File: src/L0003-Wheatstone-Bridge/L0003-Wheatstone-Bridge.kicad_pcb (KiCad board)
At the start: 2 copper layers, 64.3 x 19.3 mm, 21 parts, among them P1 12V, P2 SULLINS_PPTC041LFBN-RC, P3 CON_39299043, P4 CON_39299043, U1 MCP1703T-4002E_DB

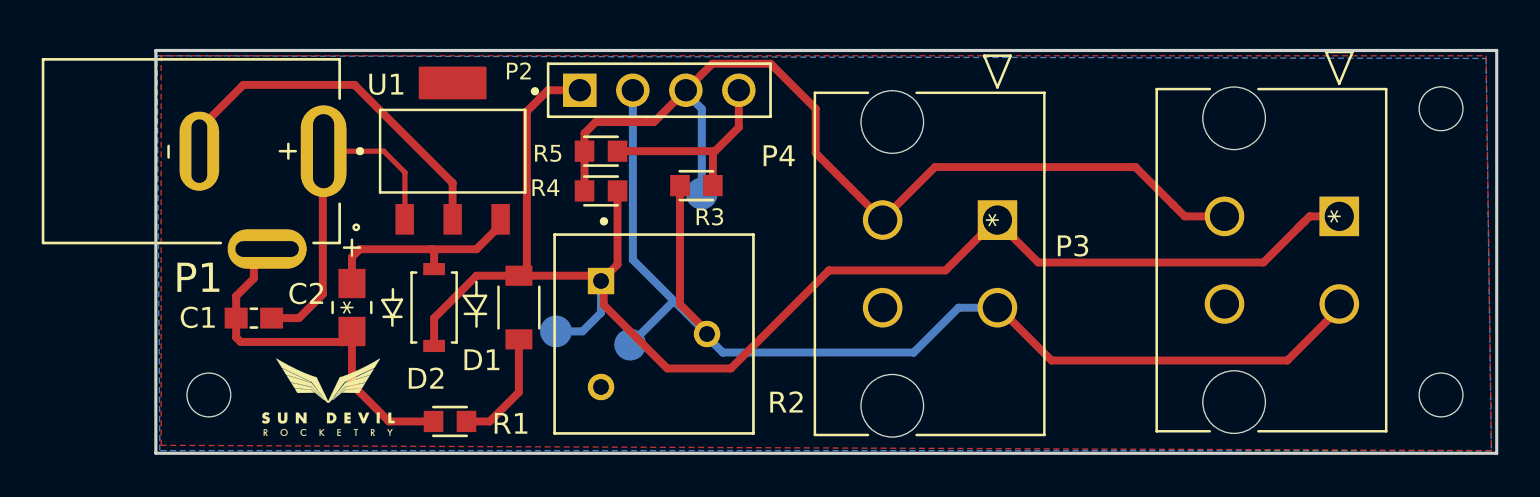
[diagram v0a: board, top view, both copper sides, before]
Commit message: routed rev 3
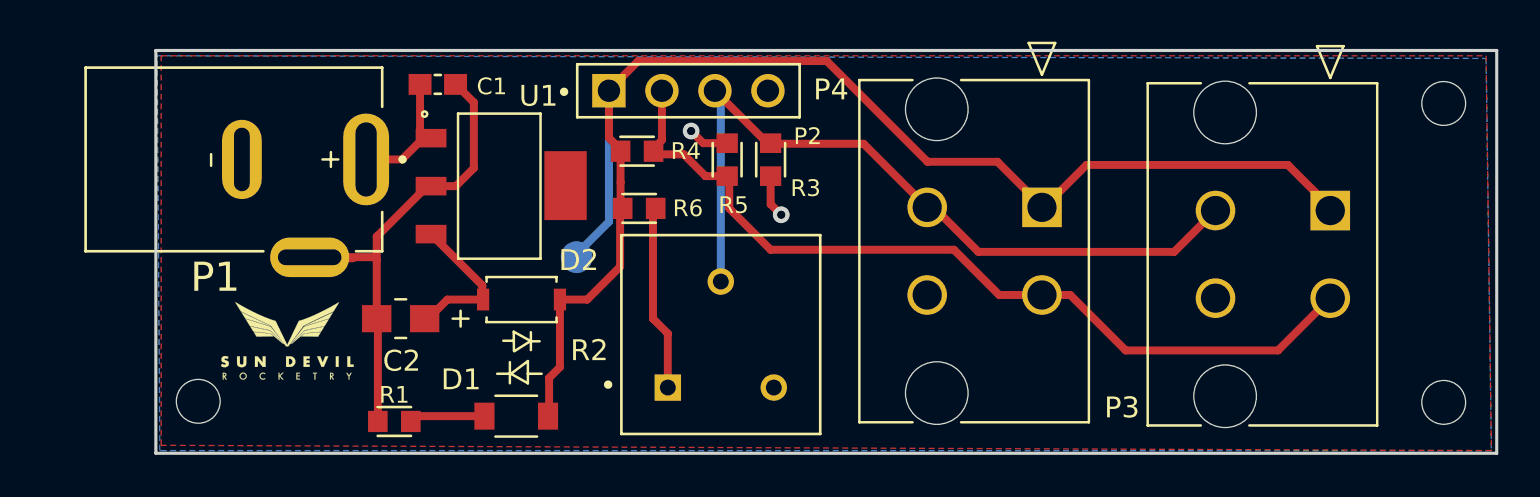
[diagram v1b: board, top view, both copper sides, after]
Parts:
- removed TP2: TP2, L0003-Wheatstone-Bridge:TP
- removed TP3: TP3, L0003-Wheatstone-Bridge:TP
- added R6: 12k, L0003-Wheatstone-Bridge:RES_0603, F.Cu at (118.4, 83.8)
- D2: value SOD-123FL_MCC -> SM5819PL-TP
- P1: value 12V -> EJ508A
- P2: value SULLINS_PPTC041LFBN-RC -> PPTC041LFBN-RC
- R3, R5: value 39k -> 12k
- R4: value 1k -> 12k
- moved H3 60.8 mm to (157.0, 78.7)
- moved H1 59.6 mm to (97.3, 93.0)
- moved C1 14.3 mm to (108.8, 77.8)
- moved H2 14.1 mm to (157.0, 93.1)
- moved R5 6.06 mm to (122.6, 81.4), turned to -90 degrees
- moved D1 5.21 mm to (112.5, 93.7), turned to 0 degrees
- moved D2 4.21 mm to (112.8, 88.1), turned to 180 degrees
- moved R3 3.77 mm to (124.7, 81.4), turned to 90 degrees
- moved TP1 3.69 mm to (115.4, 86.1)
- moved LOGO1 3.34 mm to (101.5, 90.0)
- moved R2 3.20 mm to (122.3, 89.8), turned to 0 degrees
- moved U1 2.79 mm to (111.7, 82.7), turned to -90 degrees
- moved R1 2.67 mm to (106.7, 94.0), turned to 0 degrees
- moved R4 2.57 mm to (118.3, 81.0)
- moved C2 2.40 mm to (107.0, 89.1), turned to 180 degrees
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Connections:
- C1 pad 1: Earth -> Net-(C1-Pad1)
- C1 pad 2: Net-(C1-Pad2) -> Earth
- P1 pad 1: Net-(C1-Pad2) -> Net-(C1-Pad1)
- R1 pad 1: Net-(D1-Pad1) -> Earth
- R1 pad 2: Earth -> Net-(D1-Pad1)
- R2 pad 1: +5V -> Net-(R2-Pad1)
- R2 pad 2: Vout+ -> Vout-
- R3 pad 1: Vout+ -> Earth
- R3 pad 2: Earth -> Vout-
- R4 pad 1: +5V -> Vout+
- R4 pad 2: Vout- -> +5V
- R5 pad 1: Vout- -> Earth
- R5 pad 2: Earth -> Vout+
- U1 pad 1: Net-(C1-Pad2) -> Net-(C1-Pad1)
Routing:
- net Net-(C1-Pad2): track 16.4 -> 0.00 mm
- net Vout+: track 56.9 -> 41.1 mm
- net Earth: track 43.4 -> 28.0 mm, vias 0 -> 2
- net Vout-: track 45.8 -> 36.6 mm
- net Net-(R2-Pad1): track 0.00 -> 8.88 mm
- net +5V: track 71.4 -> 65.7 mm
- net Net-(C1-Pad1): track 0.00 -> 5.53 mm
- net Net-(C2-Pad1): track 9.83 -> 6.70 mm
- net Net-(D1-Pad1): track 5.66 -> 3.45 mm
